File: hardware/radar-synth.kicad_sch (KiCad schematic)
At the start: 5 parts

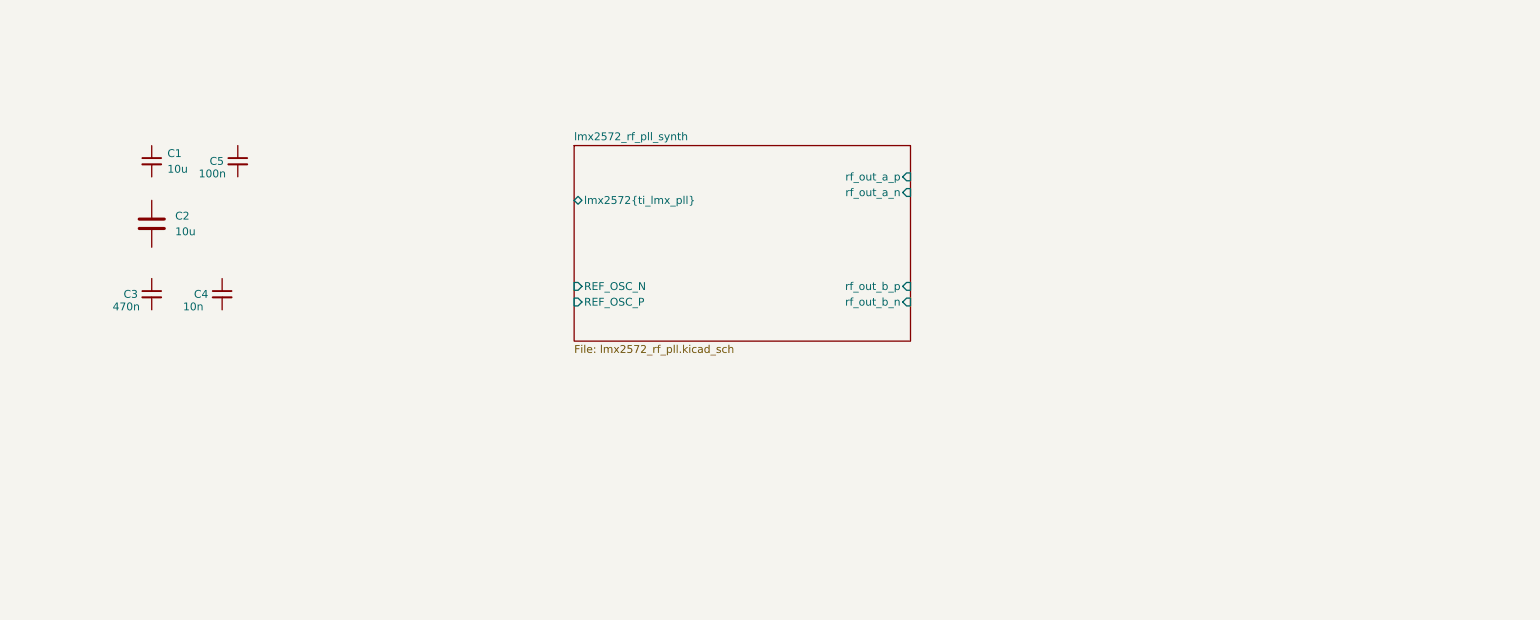
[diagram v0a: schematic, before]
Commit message: Completed schematics
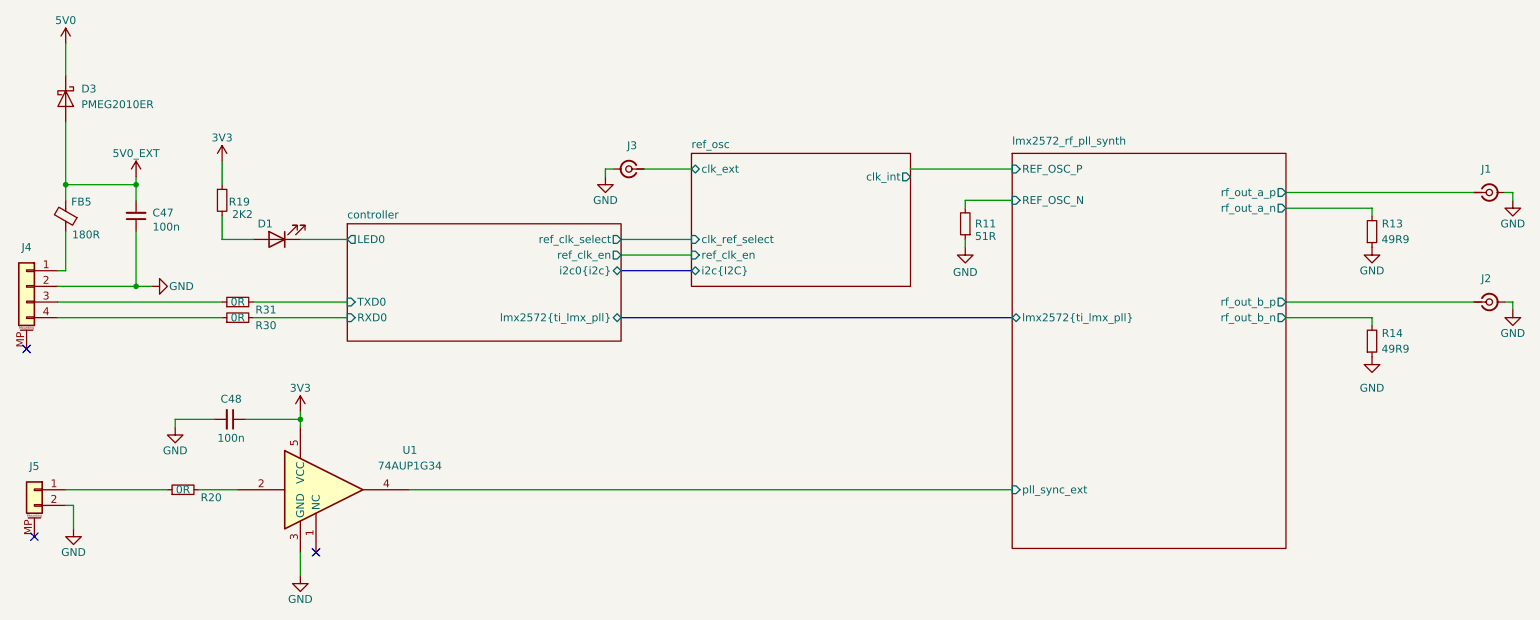
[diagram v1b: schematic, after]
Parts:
- removed C1: 10u, Capacitor_SMD:C_0603_1608Metric, symbol Device:C_Small
- removed C2: 10u, Capacitor_SMD:C_0805_2012Metric, symbol Device:C
- removed C3: 470n, Capacitor_SMD:C_0603_1608Metric, symbol Device:C_Small
- removed C4: 10n, Capacitor_SMD:C_0402_1005Metric, symbol Device:C_Small
- removed C5: 100n, Capacitor_SMD:C_0402_1005Metric, symbol Device:C_Small
- added C47, C48: 100n, Capacitor_SMD:C_0402_1005Metric, symbol Device:C_Small
- added D1: LED, LED_SMD:LED_0603_1608Metric, symbol Device:LED
- added D3: PMEG2010ER, Diode_SMD:Nexperia_CFP3_SOD-123W, symbol Diode:PMEG2010ER
- added FB5: 180R, Inductor_SMD:L_0402_1005Metric, symbol Device:FerriteBead_Small
- added J1, J2, J3: Conn_Coaxial_Small, Connector_Coaxial:SMA_Molex_73251-2120_EdgeMount_Horizontal, symbol Connector:Conn_Coaxial_Small
- added J4: Conn_01x04_MountingPin, symbol Connector_Generic_MountingPin:Conn_01x04_MountingPin
- added J5: Conn_01x02_MountingPin, symbol Connector_Generic_MountingPin:Conn_01x02_MountingPin
- added R11: 51R, Resistor_SMD:R_0402_1005Metric, symbol Device:R_Small
- added R13, R14: 49R9, Resistor_SMD:R_0402_1005Metric, symbol Device:R_Small
- added R19: 2K2, Resistor_SMD:R_0402_1005Metric, symbol Device:R_Small
- added R20, R30, R31: 0R, Resistor_SMD:R_0402_1005Metric, symbol Device:R_Small
- added U1: 74AUP1G34, symbol 74xGxx:74AUP1G34
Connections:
- net lmx2572_rf_pll_synth/REF_OSC_N: now also R11.2
- net lmx2572_rf_pll_synth/rf_out_a_n: now also R13.2
- net lmx2572_rf_pll_synth/rf_out_a_p: now also J1.1 (In)
- net lmx2572_rf_pll_synth/rf_out_b_n: now also R14.2
- net lmx2572_rf_pll_synth/rf_out_b_p: now also J2.1 (In)
- new net: J4.3 (Pin_3), R31.1
- new net: R20.2, U1.2
- new net: J4.4 (Pin_4), R30.1
- new net: J5.1 (Pin_1), R20.1
- new net: FB5.1, J4.1 (Pin_1)
- new net: D1.2 (A), R19.2
- new net 3V3: C48.1, R19.1, U1.5 (VCC)
- new net 5V0: D3.1 (K)
- new net 5V0_EXT: C47.2, D3.2 (A), FB5.2
- new net GND: C47.1, C48.2, J1.2 (Ext), J2.2 (Ext), J3.2 (Ext), J4.2 (Pin_2), J5.2 (Pin_2), R11.1, R13.1, R14.1, U1.3 (GND)
- new net controller/LED0: D1.1 (K)
- new net controller/RXD0: R30.2
- new net controller/TXD0: R31.2
- new net lmx2572_rf_pll_synth/pll_sync_ext: U1.4
- new net ref_osc/clk_ext: J3.1 (In)
- no-connect marks 0 -> 3
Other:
- added sheet controller (xia0_esp32s3p_controller.kicad_sch)
- added sheet ref_osc (reference_clock.kicad_sch)
- sheet lmx2572_rf_pll_synth ports: added pll_sync_ext; removed none
- company: (none) -> ${COMPANY}
- title: (none) -> TOP LEVEL
